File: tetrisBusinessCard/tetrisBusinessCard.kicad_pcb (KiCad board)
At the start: 2 copper layers, 48.7 x 84.5 mm, 497 parts, among them SW1 SW_Push, SW2 SW_Push, SW3 SW_Push, SW4 SW_Push, SW5 SW_Push, SW6 SW_Push, SW7 SW_DPST_x2, U1 SC091413, U2 W25Q16JVUXIQ, Y1 ABMB-272-T3

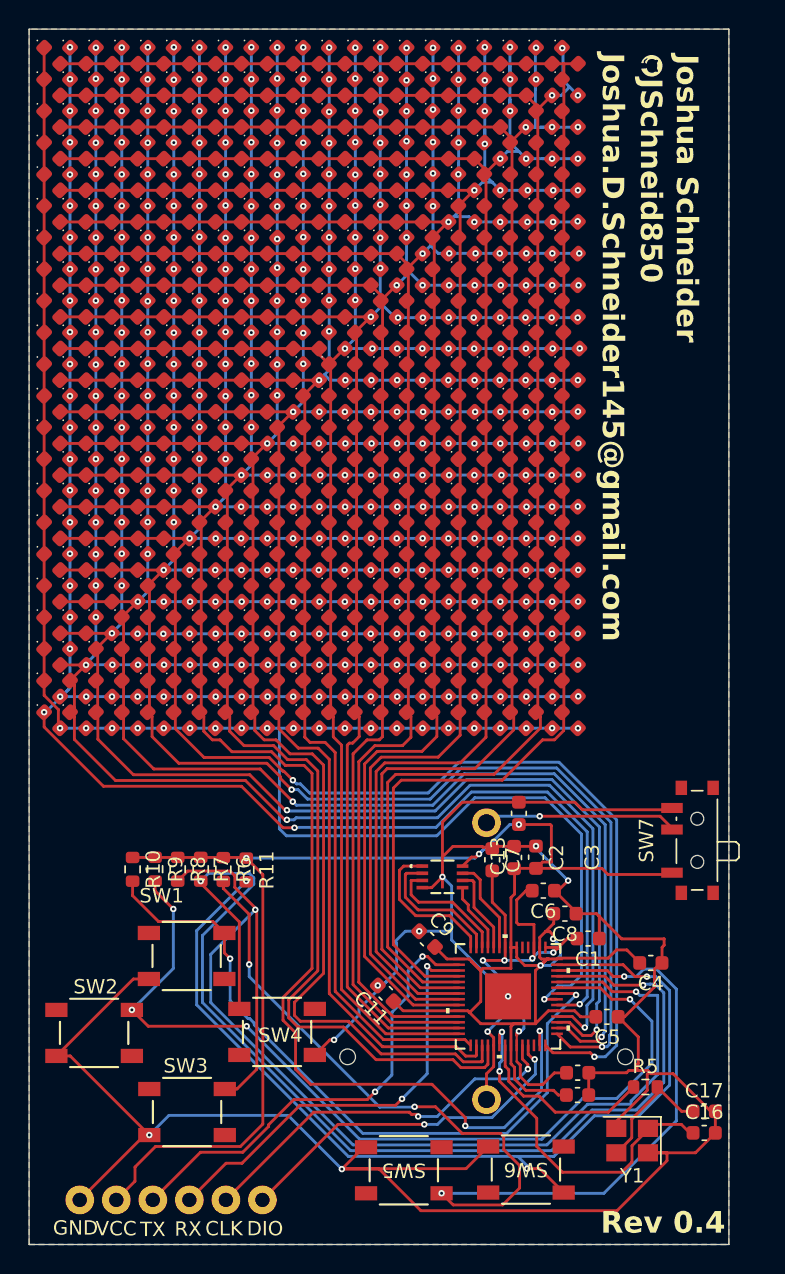
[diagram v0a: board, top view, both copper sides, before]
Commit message: Fully Working Card. In need of a re-factor though I dont know what compelled me to not use .h files
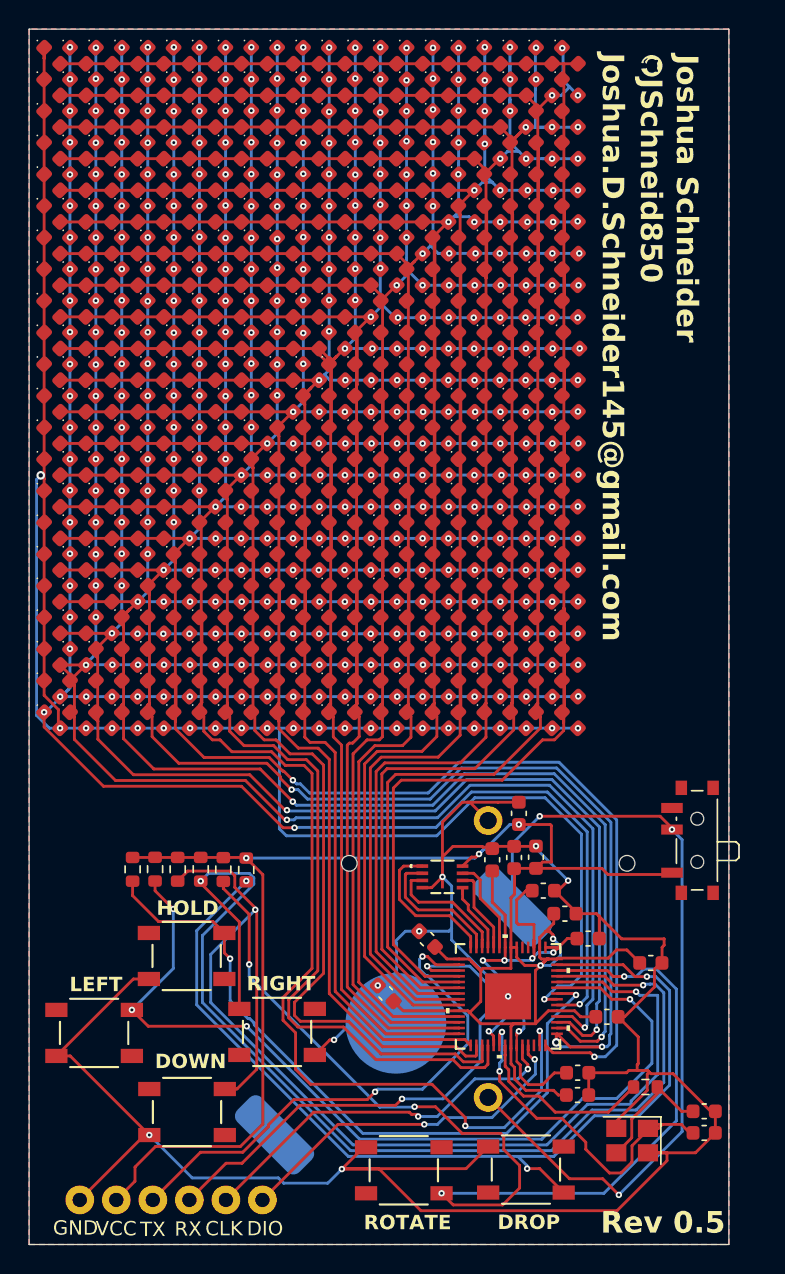
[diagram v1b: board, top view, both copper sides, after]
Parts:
- added QR: LOGO, MyFootprints:qrCode, B.Cu at (197.4, 42.2)
- added REF**: MYOUNG MY-2032-12, MyFootprints:MYOUNG MY-2032-12, F.Cu at (198.7, 88.9)
- moved B1 19.1 mm to (205.1, 94.0), turned to 0 degrees
- renumbered G*** to Github
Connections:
- SW7 pad 3: GND -> (no net)
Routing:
- net Net-(SW7A-B): track 13.1 -> 58.3 mm, vias 1 -> 3
- net CHRLY_2: track 112.5 -> 145.1 mm
- net CHRLY_1: track 112.0 -> 140.0 mm
- net CHRLY_3: track 113.6 -> 135.3 mm
- net CHRLY_6: track 112.2 -> 132.9 mm
- net CHRLY_22: track 127.9 -> 148.4 mm, vias 22 -> 23
- net CHRLY_9: track 111.1 -> 129.5 mm
- net CHRLY_5: track 112.6 -> 129.0 mm
- net CHRLY_8: track 111.0 -> 125.7 mm
- net CHRLY_10: track 111.1 -> 125.1 mm
- net GND: track 190.7 -> 176.8 mm
- net CHRLY_7: track 111.1 -> 124.6 mm
- net CHRLY_4: track 114.0 -> 122.7 mm
- net CHRLY_11: track 114.2 -> 122.9 mm
- net RX: track 30.0 -> 37.6 mm
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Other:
- board text added: "DOWN"
- board text added: "DROP"
- board text added: "HOLD"
- board text added: "LEFT"
- board text added: "RIGHT"
- board text added: "ROTATE"
- board text added: "Rev 0.5"
- board text removed: "Rev 0.4"
